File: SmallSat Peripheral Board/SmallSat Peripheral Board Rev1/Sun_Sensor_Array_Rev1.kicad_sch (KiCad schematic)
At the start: 16 parts

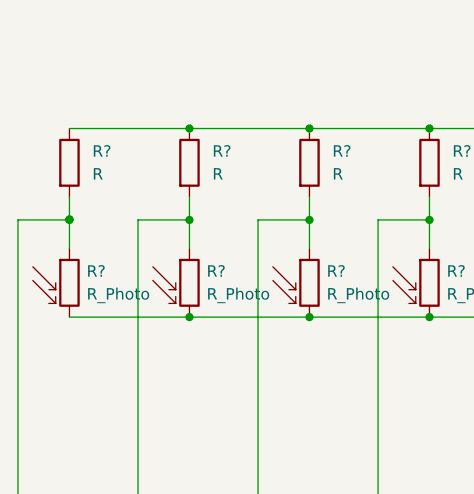
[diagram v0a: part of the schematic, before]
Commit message: PB-order version
Sent the order in for Rev 1 power board with this version
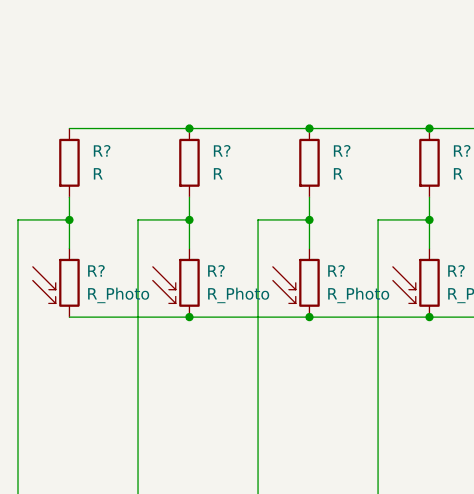
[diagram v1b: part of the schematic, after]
